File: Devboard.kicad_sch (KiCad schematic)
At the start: 30 parts, among them J1 USB_C_Receptacle_USB2.0_14P, SW1 SW_Push, U1 RP2040, U2 NCP1117-3.3_SOT223, U3 W25Q128JVS, Y1 12 MHz

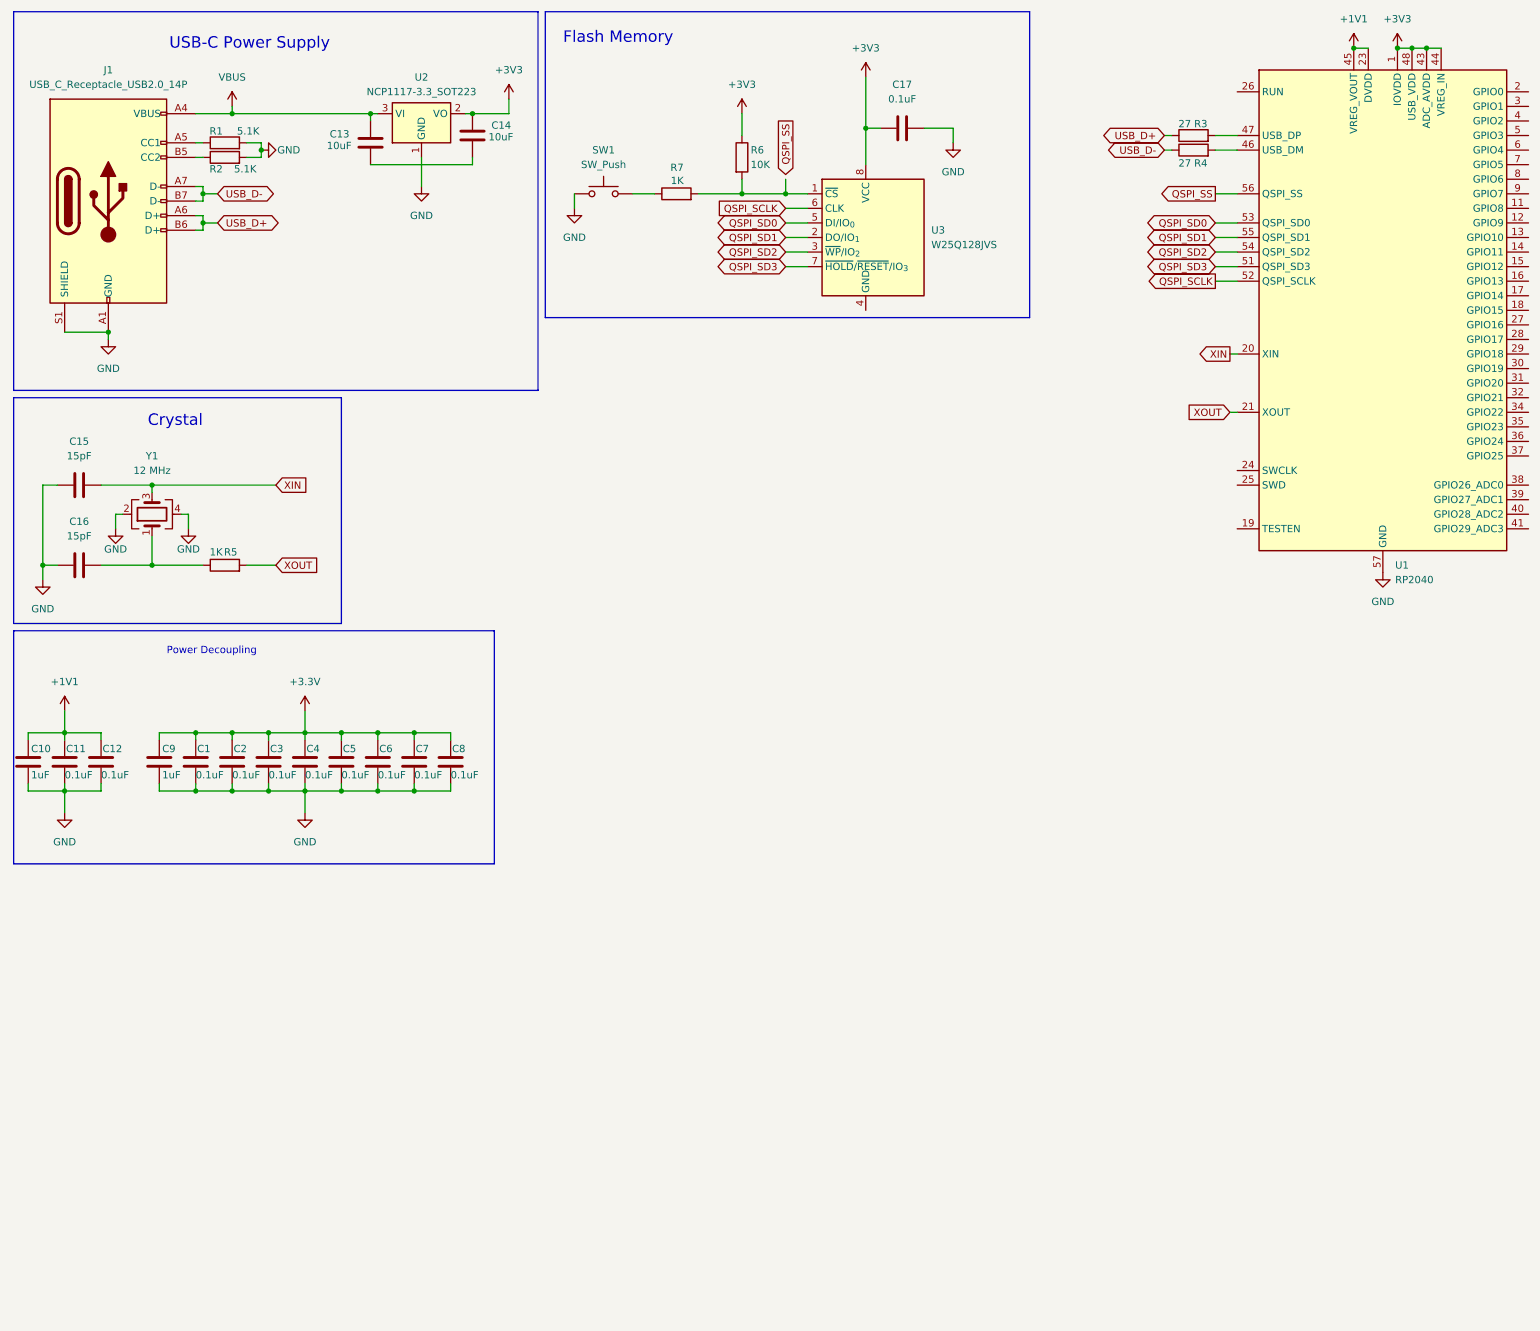
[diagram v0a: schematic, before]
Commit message: Actually finished schematic
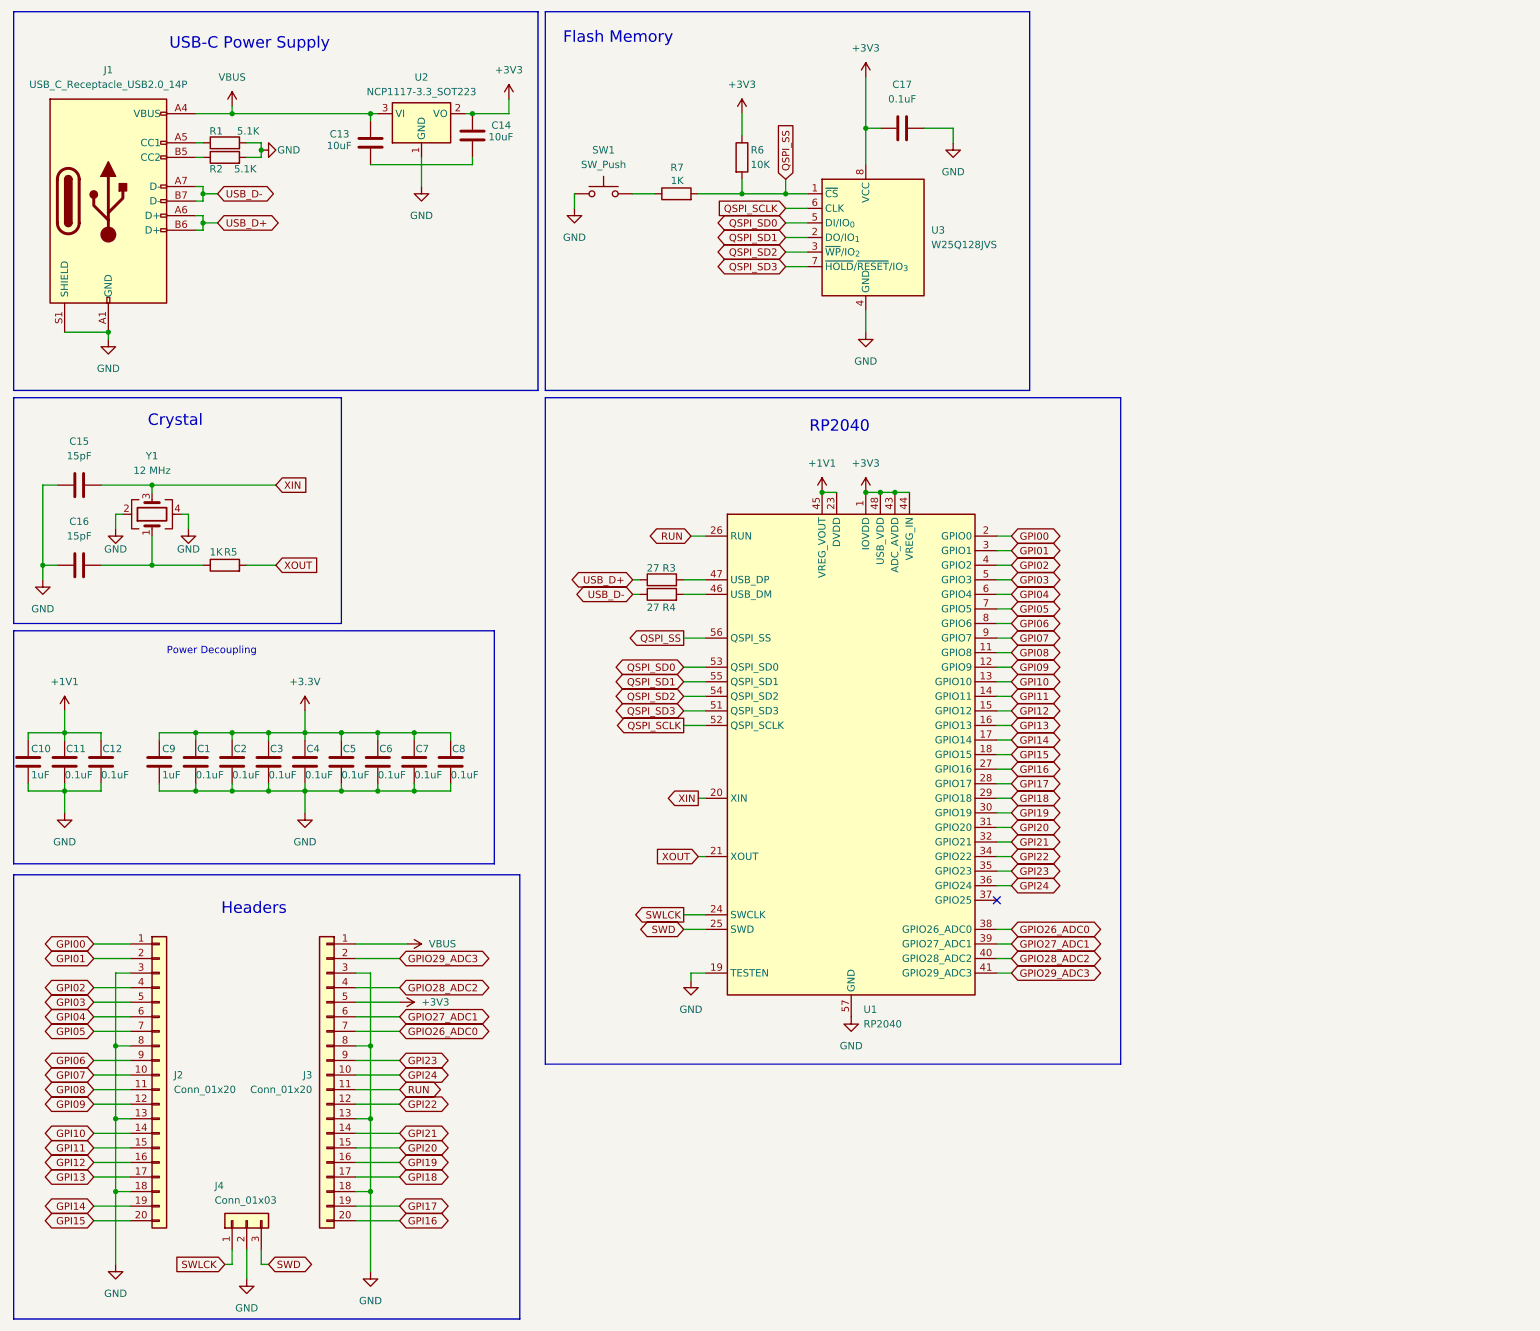
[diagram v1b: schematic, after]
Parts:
- added J2, J3: Conn_01x20, symbol Connector_Generic:Conn_01x20
- added J4: Conn_01x03, symbol Connector_Generic:Conn_01x03
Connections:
- net +3V3: now also J3.5 (Pin_5)
- net GND: now also U1.19 (TESTEN), U3.4 (GND), J2.13 (Pin_13), J2.18 (Pin_18), J2.3 (Pin_3), J2.8 (Pin_8), J3.13 (Pin_13), J3.18 (Pin_18), J3.3 (Pin_3), J3.8 (Pin_8), J4.2 (Pin_2)
- net QSPI_SS: now also R6.2, R7.2, U3.1 (~{CS})
- net VBUS: now also J3.1 (Pin_1)
- net GPI08: now reaches U1.11 (GPIO8)
- net GPI08: now also J2.11 (Pin_11)
- net GPI09: now reaches U1.12 (GPIO9)
- net GPI09: now also J2.12 (Pin_12)
- net GPI10: now reaches U1.13 (GPIO10)
- net GPI10: now also J2.14 (Pin_14)
- net GPI11: now reaches U1.14 (GPIO11)
- net GPI11: now also J2.15 (Pin_15)
- net GPI12: now reaches U1.15 (GPIO12)
- net GPI12: now also J2.16 (Pin_16)
- net GPI13: now reaches U1.16 (GPIO13)
- net GPI13: now also J2.17 (Pin_17)
- net GPI14: now reaches U1.17 (GPIO14)
- net GPI14: now also J2.19 (Pin_19)
- net GPI15: now reaches U1.18 (GPIO15)
- net GPI15: now also J2.20 (Pin_20)
- net GPI00: now reaches U1.2 (GPIO0)
- net GPI00: now also J2.1 (Pin_1)
- net SWLCK: now reaches U1.24 (SWCLK)
- net SWLCK: now also J4.1 (Pin_1)
- net SWD: now reaches U1.25 (SWD)
- net SWD: now also J4.3 (Pin_3)
- net RUN: now reaches U1.26 (RUN)
- net RUN: now also J3.11 (Pin_11)
- net GPI16: now reaches U1.27 (GPIO16)
- net GPI16: now also J3.20 (Pin_20)
- net GPI17: now reaches U1.28 (GPIO17)
- net GPI17: now also J3.19 (Pin_19)
- net GPI18: now reaches U1.29 (GPIO18)
- net GPI18: now also J3.17 (Pin_17)
- net GPI01: now reaches U1.3 (GPIO1)
- net GPI01: now also J2.2 (Pin_2)
- net GPI19: now reaches U1.30 (GPIO19)
- net GPI19: now also J3.16 (Pin_16)
- net GPI20: now reaches U1.31 (GPIO20)
- net GPI20: now also J3.15 (Pin_15)
- net GPI21: now reaches U1.32 (GPIO21)
- net GPI21: now also J3.14 (Pin_14)
- net GPI22: now reaches U1.34 (GPIO22)
- net GPI22: now also J3.12 (Pin_12)
- net GPI23: now reaches U1.35 (GPIO23)
- net GPI23: now also J3.9 (Pin_9)
- net GPI24: now reaches U1.36 (GPIO24)
- net GPI24: now also J3.10 (Pin_10)
- net GPIO26_ADC0: now reaches U1.38 (GPIO26_ADC0)
- net GPIO26_ADC0: now also J3.7 (Pin_7)
- net GPIO27_ADC1: now reaches U1.39 (GPIO27_ADC1)
- net GPIO27_ADC1: now also J3.6 (Pin_6)
- net GPI02: now reaches U1.4 (GPIO2)
- net GPI02: now also J2.4 (Pin_4)
- net GPIO28_ADC2: now reaches U1.40 (GPIO28_ADC2)
- net GPIO28_ADC2: now also J3.4 (Pin_4)
- net GPIO29_ADC3: now reaches U1.41 (GPIO29_ADC3)
- net GPIO29_ADC3: now also J3.2 (Pin_2)
- net GPI03: now reaches U1.5 (GPIO3)
- net GPI03: now also J2.5 (Pin_5)
- net GPI04: now reaches U1.6 (GPIO4)
- net GPI04: now also J2.6 (Pin_6)
- net GPI05: now reaches U1.7 (GPIO5)
- net GPI05: now also J2.7 (Pin_7)
- net GPI06: now reaches U1.8 (GPIO6)
- net GPI06: now also J2.9 (Pin_9)
- net GPI07: now reaches U1.9 (GPIO7)
- net GPI07: now also J2.10 (Pin_10)
- no-connect marks 0 -> 1
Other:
- note added: "Headers"
- note added: "RP2040"
- moved on the sheet: R3, R4, U1
